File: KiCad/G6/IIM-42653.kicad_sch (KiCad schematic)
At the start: 8 parts, among them U10 IIM-42653, U11 IIM-42653

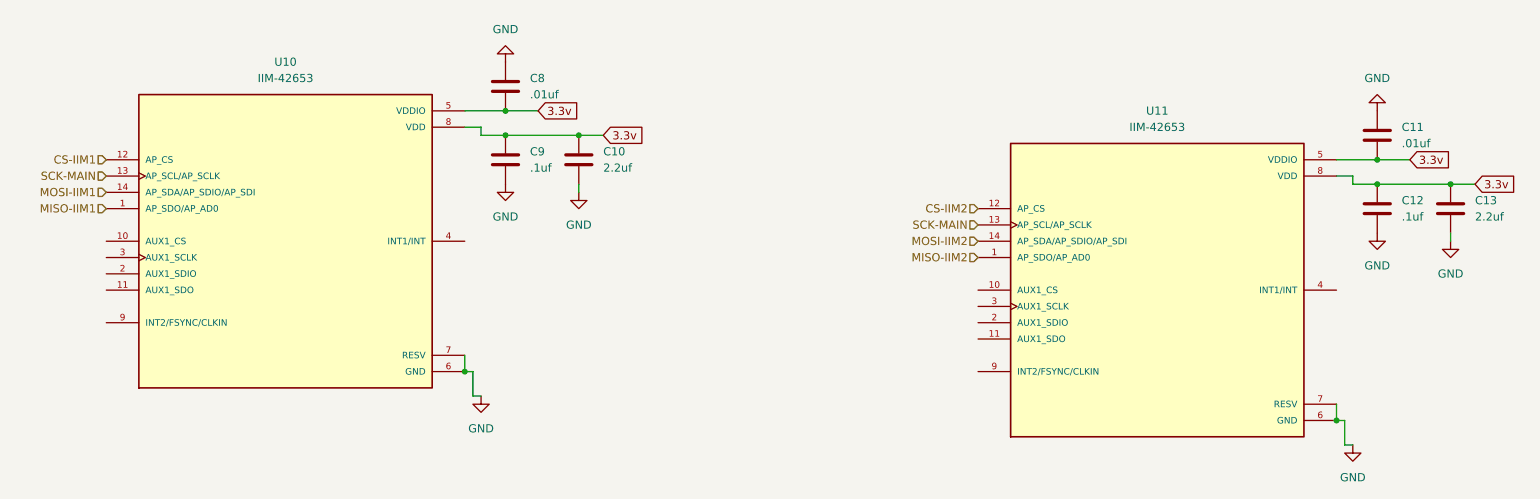
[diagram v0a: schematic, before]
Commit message: g6
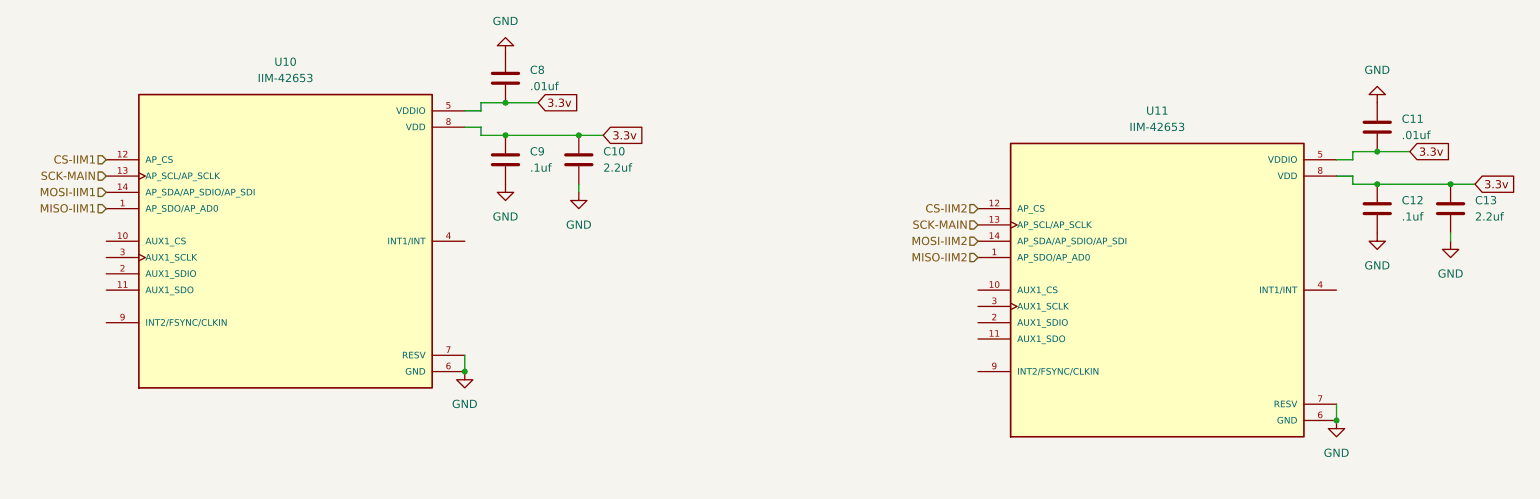
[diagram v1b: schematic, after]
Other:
- moved on the sheet: C11, C8
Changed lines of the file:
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@@
 	)
 	(junction
-		(at 106.68 80.01)
+		(at 106.68 78.74)
 		(diameter 0)
 		(color 0 0 0 0)
@@
 	)
 	(junction
-		(at 242.57 87.63)
+		(at 242.57 86.36)
 		(diameter 0)
 		(color 0 0 0 0)
@@
 	(wire
 		(pts
-			(xy 237.49 132.08) (xy 237.49 128.27)
-		)
-		(stroke
-			(width 0)
-			(type default)
-		)
-	)
-	(wire
-		(pts
-			(xy 238.76 132.08) (xy 237.49 132.08)
-		)
-		(stroke
-			(width 0)
-			(type default)
-		)
-	)
-	(wire
-		(pts
-			(xy 242.57 87.63) (xy 247.65 87.63)
-		)
-		(stroke
-			(width 0)
-			(type default)
-		)
-	)
-	(wire
-		(pts
-			(xy 101.6 120.65) (xy 100.33 120.65)
-		)
-		(stroke
-			(width 0)
-			(type default)
-		)
-	)
-	(wire
-		(pts
-			(xy 106.68 80.01) (xy 111.76 80.01)
-		)
-		(stroke
-			(width 0)
-			(type default)
-		)
-	)
-	(wire
-		(pts
-			(xy 236.22 87.63) (xy 242.57 87.63)
+			(xy 102.87 80.01) (xy 100.33 80.01)
+		)
+		(stroke
+			(width 0)
+			(type default)
+		)
+	)
+	(wire
+		(pts
+			(xy 238.76 86.36) (xy 238.76 87.63)
+		)
+		(stroke
+			(width 0)
+			(type default)
+		)
+	)
+	(wire
+		(pts
+			(xy 242.57 86.36) (xy 247.65 86.36)
+		)
+		(stroke
+			(width 0)
+			(type default)
+		)
+	)
+	(wire
+		(pts
+			(xy 106.68 78.74) (xy 111.76 78.74)
+		)
+		(stroke
+			(width 0)
+			(type default)
+		)
+	)
+	(wire
+		(pts
+			(xy 238.76 86.36) (xy 242.57 86.36)
 		)
 		(stroke
@@
 	(wire
 		(pts
-			(xy 102.87 124.46) (xy 101.6 124.46)
-		)
-		(stroke
-			(width 0)
-			(type default)
-		)
-	)
-	(wire
-		(pts
-			(xy 237.49 128.27) (xy 236.22 128.27)
+			(xy 102.87 78.74) (xy 102.87 80.01)
+		)
+		(stroke
+			(width 0)
+			(type default)
+		)
+	)
+	(wire
+		(pts
+			(xy 238.76 87.63) (xy 236.22 87.63)
 		)
 		(stroke
@@
 	(wire
 		(pts
-			(xy 101.6 124.46) (xy 101.6 120.65)
-		)
-		(stroke
-			(width 0)
-			(type default)
-		)
-	)
-	(wire
-		(pts
-			(xy 100.33 80.01) (xy 106.68 80.01)
+			(xy 102.87 78.74) (xy 106.68 78.74)
 		)
 		(stroke
@@
 	(global_label "3.3v"
 		(shape input)
-		(at 247.65 87.63 0)
+		(at 247.65 86.36 0)
 		(fields_autoplaced yes)
 		(effects
@@
 		)
 		(property "Intersheetrefs" "${INTERSHEET_REFS}"
-			(at 254.6266 87.63 0)
+			(at 254.6266 86.36 0)
 			(effects
 				(font
@@
 	(global_label "3.3v"
 		(shape input)
-		(at 111.76 80.01 0)
+		(at 111.76 78.74 0)
 		(fields_autoplaced yes)
 		(effects
@@
 		)
 		(property "Intersheetrefs" "${INTERSHEET_REFS}"
-			(at 118.7366 80.01 0)
+			(at 118.7366 78.74 0)
 			(effects
 				(font
@@
 	(symbol
 		(lib_id "Device:C")
-		(at 106.68 76.2 0)
+		(at 106.68 74.93 0)
 		(unit 1)
 		(exclude_from_sim no)
@@
 		(fields_autoplaced yes)
 		(property "Reference" "C8"
-			(at 110.49 74.9299 0)
+			(at 110.49 73.6599 0)
 			(effects
 				(font
@@
 		)
 		(property "Value" ".01uf"
-			(at 110.49 77.4699 0)
+			(at 110.49 76.1999 0)
 			(effects
 				(font
@@
 		)
 		(property "Footprint" "CC0603KRXQRQBB104:.01YAG_CC1206_YAG"
-			(at 107.6452 80.01 0)
+			(at 107.6452 78.74 0)
 			(effects
 				(font
@@
 		)
 		(property "Datasheet" "~"
-			(at 106.68 76.2 0)
+			(at 106.68 74.93 0)
 			(effects
 				(font
@@
 		)
 		(property "Description" "Unpolarized capacitor"
-			(at 106.68 76.2 0)
+			(at 106.68 74.93 0)
 			(effects
 				(font
@@
 	(symbol
 		(lib_id "power:GND")
-		(at 238.76 132.08 0)
+		(at 236.22 128.27 0)
 		(unit 1)
 		(exclude_from_sim no)
@@
 		(fields_autoplaced yes)
 		(property "Reference" "#PWR039"
-			(at 238.76 138.43 0)
+			(at 236.22 134.62 0)
 			(effects
 				(font
@@
 		)
 		(property "Value" "GND"
-			(at 238.76 137.16 0)
+			(at 236.22 133.35 0)
 			(effects
 				(font
@@
 		)
 		(property "Footprint" ""
-			(at 238.76 132.08 0)
+			(at 236.22 128.27 0)
 			(effects
 				(font
@@
 		)
 		(property "Datasheet" ""
-			(at 238.76 132.08 0)
+			(at 236.22 128.27 0)
 			(effects
 				(font
@@
 		)
 		(property "Description" "Power symbol creates a global label with name \"GND\" , ground"
-			(at 238.76 132.08 0)
+			(at 236.22 128.27 0)
 			(effects
 				(font
@@
 	(symbol
 		(lib_id "Device:C")
-		(at 242.57 83.82 0)
+		(at 242.57 82.55 0)
 		(unit 1)
 		(exclude_from_sim no)
@@
 		(fields_autoplaced yes)
 		(property "Reference" "C11"
-			(at 246.38 82.5499 0)
+			(at 246.38 81.2799 0)
 			(effects
 				(font
@@
 		)
 		(property "Value" ".01uf"
-			(at 246.38 85.0899 0)
+			(at 246.38 83.8199 0)
 			(effects
 				(font
@@
 		)
 		(property "Footprint" "CC0603KRXQRQBB104:.01YAG_CC1206_YAG"
-			(at 243.5352 87.63 0)
+			(at 243.5352 86.36 0)
 			(effects
 				(font
@@
 		)
 		(property "Datasheet" "~"
-			(at 242.57 83.82 0)
+			(at 242.57 82.55 0)
 			(effects
 				(font
@@
 		)
 		(property "Description" "Unpolarized capacitor"
-			(at 242.57 83.82 0)
+			(at 242.57 82.55 0)
 			(effects
 				(font
@@
 	(symbol
 		(lib_id "power:GND")
-		(at 242.57 80.01 180)
+		(at 242.57 78.74 180)
 		(unit 1)
 		(exclude_from_sim no)
@@
 		(fields_autoplaced yes)
 		(property "Reference" "#PWR044"
+			(at 242.57 72.39 0)
+			(effects
+				(font
+					(size 1.27 1.27)
+				)
+				(hide yes)
+			)
+		)
+		(property "Value" "GND"
 			(at 242.57 73.66 0)
 			(effects
@@
 					(size 1.27 1.27)
 				)
-				(hide yes)
-			)
-		)
-		(property "Value" "GND"
-			(at 242.57 74.93 0)
-			(effects
-				(font
-					(size 1.27 1.27)
-				)
 			)
 		)
 		(property "Footprint" ""
-			(at 242.57 80.01 0)
+			(at 242.57 78.74 0)
 			(effects
 				(font
@@
 		)
 		(property "Datasheet" ""
-			(at 242.57 80.01 0)
+			(at 242.57 78.74 0)
 			(effects
 				(font
@@
 		)
 		(property "Description" "Power symbol creates a global label with name \"GND\" , ground"
-			(at 242.57 80.01 0)
+			(at 242.57 78.74 0)
 			(effects
 				(font
@@
 	(symbol
 		(lib_id "power:GND")
-		(at 106.68 72.39 180)
+		(at 106.68 71.12 180)
 		(unit 1)
 		(exclude_from_sim no)
@@
 		(fields_autoplaced yes)
 		(property "Reference" "#PWR040"
+			(at 106.68 64.77 0)
+			(effects
+				(font
+					(size 1.27 1.27)
+				)
+				(hide yes)
+			)
+		)
+		(property "Value" "GND"
 			(at 106.68 66.04 0)
 			(effects
@@
 					(size 1.27 1.27)
 				)
-				(hide yes)
-			)
-		)
-		(property "Value" "GND"
-			(at 106.68 67.31 0)
-			(effects
-				(font
-					(size 1.27 1.27)
-				)
 			)
 		)
 		(property "Footprint" ""
-			(at 106.68 72.39 0)
+			(at 106.68 71.12 0)
 			(effects
 				(font
@@
 		)
 		(property "Datasheet" ""
-			(at 106.68 72.39 0)
+			(at 106.68 71.12 0)
 			(effects
 				(font
@@
 		)
 		(property "Description" "Power symbol creates a global label with name \"GND\" , ground"
-			(at 106.68 72.39 0)
+			(at 106.68 71.12 0)
 			(effects
 				(font
@@
 	(symbol
 		(lib_id "power:GND")
-		(at 102.87 124.46 0)
+		(at 100.33 120.65 0)
 		(unit 1)
 		(exclude_from_sim no)
@@
 		(fields_autoplaced yes)
 		(property "Reference" "#PWR043"
-			(at 102.87 130.81 0)
+			(at 100.33 127 0)
 			(effects
 				(font
@@
 		)
 		(property "Value" "GND"
-			(at 102.87 129.54 0)
+			(at 100.33 125.73 0)
 			(effects
 				(font
@@
 		)
 		(property "Footprint" ""
-			(at 102.87 124.46 0)
+			(at 100.33 120.65 0)
 			(effects
 				(font
@@
 		)
 		(property "Datasheet" ""
-			(at 102.87 124.46 0)
+			(at 100.33 120.65 0)
 			(effects
 				(font
@@
 		)
 		(property "Description" "Power symbol creates a global label with name \"GND\" , ground"
-			(at 102.87 124.46 0)
-			(effects
-				(font
+			(at 100.33 120.65 0)
+			(effects
+				(font
